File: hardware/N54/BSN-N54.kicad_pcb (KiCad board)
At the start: 4 copper layers, 34 x 34 mm, 46 parts, among them J1 Conn_Coaxial_Small, U1 nRF54L05-QFXX, U2 SHTC3, U3 HDC2010, X1 32MHz, X2 32.768kHz

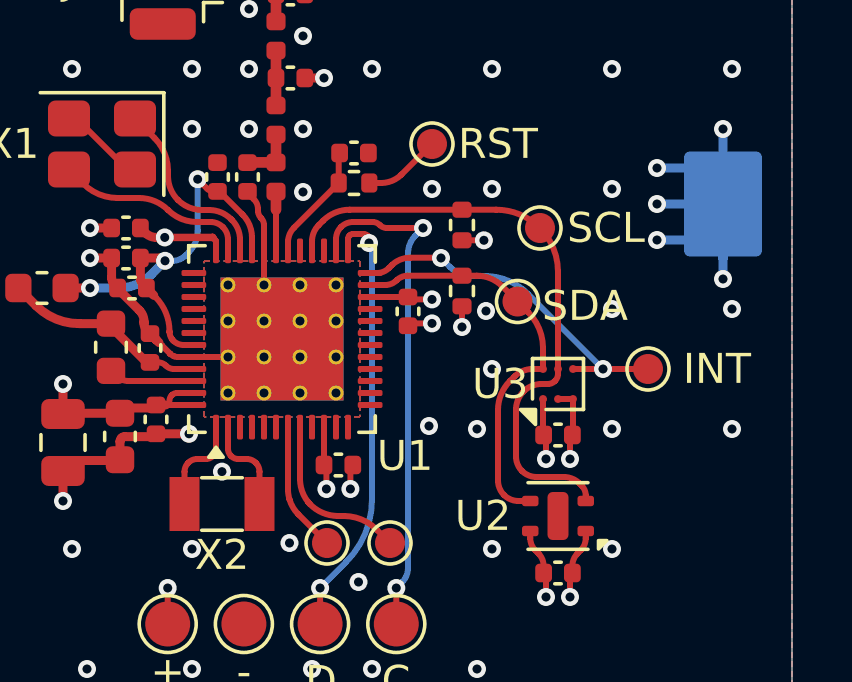
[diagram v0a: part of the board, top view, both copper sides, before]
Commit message: More small fixes & Created new panel
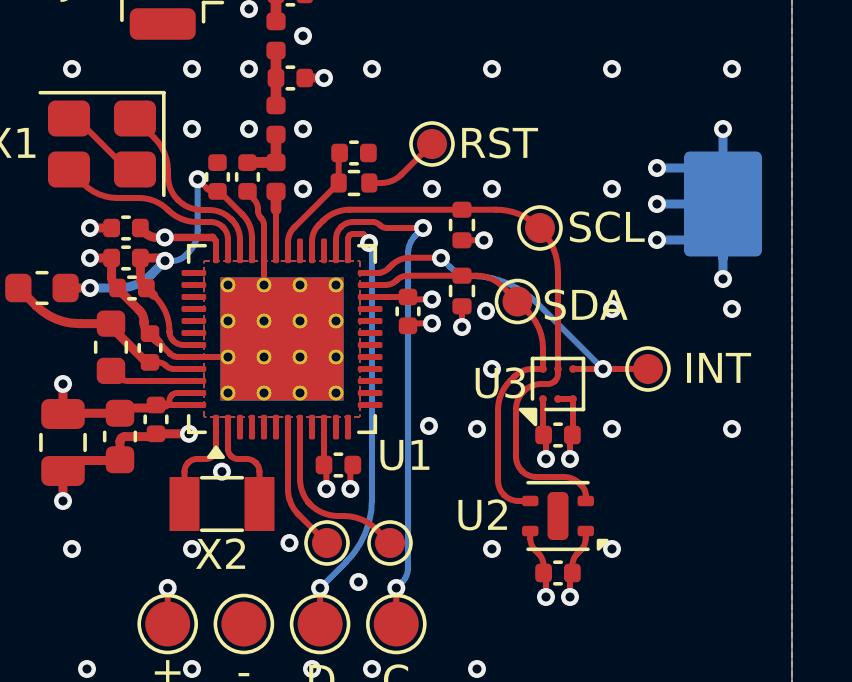
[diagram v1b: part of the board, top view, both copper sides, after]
